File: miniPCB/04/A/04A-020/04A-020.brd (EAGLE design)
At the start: 41 parts

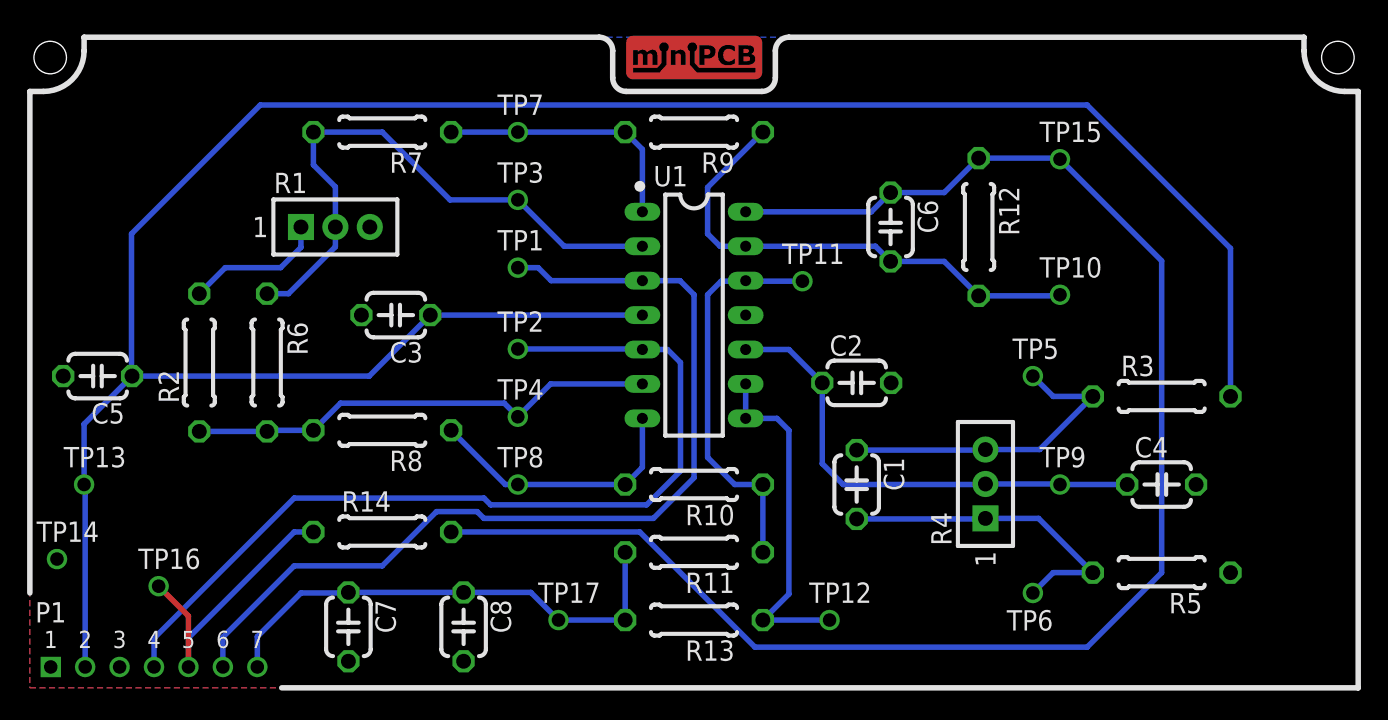
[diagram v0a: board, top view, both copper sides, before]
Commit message: NM.14JAN2023
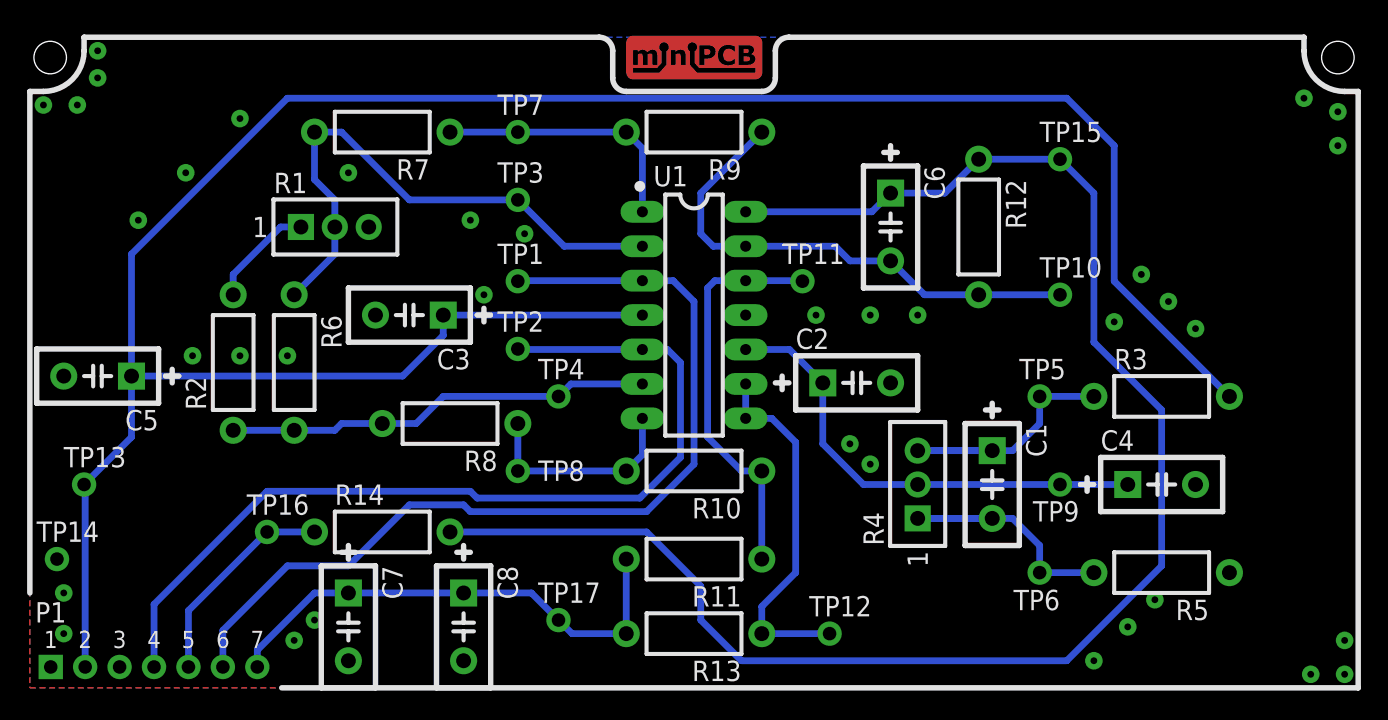
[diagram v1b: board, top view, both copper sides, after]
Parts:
- U1: value (none) -> OPAMP_QUADTHD
- moved C1 10.0 mm to (72.0, 16.0)
- moved TP16 8.94 mm to (18.5, 12.5)
- moved R8 5.02 mm to (32.0, 20.5)
- moved R4 5.00 mm to (66.5, 13.5)
- moved TP4 3.35 mm to (40.0, 22.5)
- moved R2 2.50 mm to (16.0, 25.0)
- moved R6 2.00 mm to (20.5, 25.0)
- moved TP5 1.58 mm to (75.5, 22.5)
- moved TP6 1.58 mm to (75.5, 9.50)
- moved C3 1.00 mm to (29.0, 28.5)
- moved R10 1.00 mm to (50.0, 17.0)
- moved R13 1.00 mm to (50.0, 5.00)
- moved TP1 1.00 mm to (37.0, 31.0)
- moved TP12 1.00 mm to (60.0, 5.00)
- moved TP8 1.00 mm to (37.0, 17.0)
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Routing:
- net N$11: track 21.5 -> 15.9 mm
- net N$8: track 19.9 -> 15.9 mm
- net N$6: track 35.0 -> 31.6 mm
- net POT.1: track 24.1 -> 21.3 mm
- net POT.3: track 24.1 -> 21.3 mm
- net N$10: track 10.4 -> 7.95 mm
- net OUT: track 116.7 -> 118.7 mm
- net N$5: track 43.4 -> 41.5 mm
- net N$9: track 25.8 -> 27.1 mm
- net N$4: track 69.6 -> 68.6 mm
- net N$3: track 66.9 -> 67.8 mm
- net BIAS: track 35.8 -> 35.0 mm
- net VFB: track 37.1 -> 37.7 mm
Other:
- board text added: "INSTRUMENTATION AMPLIFIER"

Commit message: NM.07MAR2024
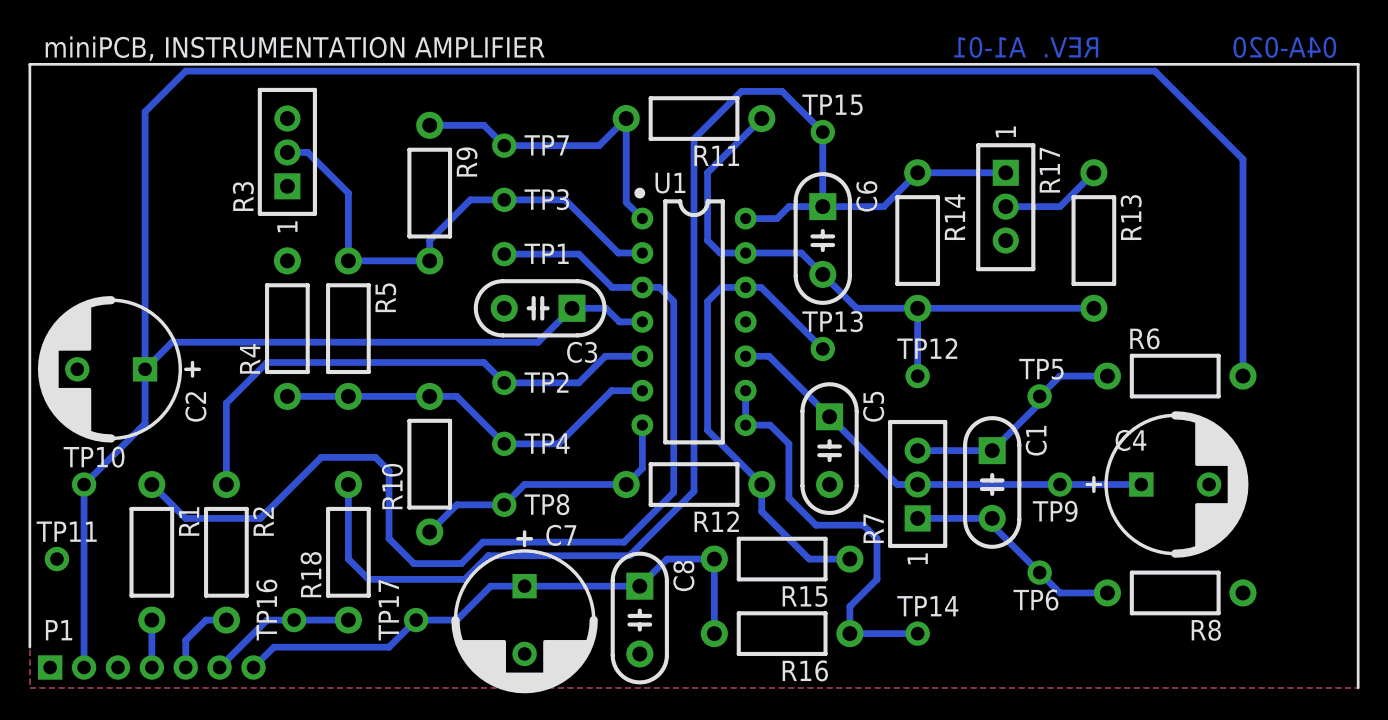
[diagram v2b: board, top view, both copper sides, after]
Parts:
- removed P1-: (no value), minipcb:MINIPCB_7P_50X100
- added P1: (no value), minipcb:PINS_1X7
- added R15, R16, R18: (no value), minipcb:0207/10
- added R17: (no value), minipcb:TRIM_0100
- added U2: CLASSIC-50X100, miniPCB_BOARDS:PCB50X100
- C2, C4, C7: device minipcb:C050-024X044 -> minipcb:C5MM
- R1, R4: device minipcb:TRIM_0100 -> minipcb:0207/10
- R3, R7: device minipcb:0207/10 -> minipcb:TRIM_0100
- U1: value OPAMP_QUADTHD -> (none)
- moved TP10 73.3 mm to (5.00, 16.0)
- moved R3 66.3 mm to (20.0, 38.0), turned to 90 degrees
- moved R6 65.0 mm to (85.5, 24.0), turned to 0 degrees
- moved TP14 63.7 mm to (66.5, 5.00)
- moved R5 62.6 mm to (24.5, 27.5), turned to 270 degrees
- moved TP11 58.7 mm to (3.00, 10.5)
- moved TP13 55.4 mm to (59.5, 26.0)
- moved C2 55.0 mm to (7.00, 24.5), turned to 180 degrees
- moved R8 54.9 mm to (85.5, 8.00)
- moved C5 54.3 mm to (60.0, 18.5), turned to 270 degrees
- moved R7 48.7 mm to (66.5, 13.5), turned to 90 degrees
- moved R4 48.6 mm to (20.0, 27.5)
- moved R14 45.0 mm to (66.5, 34.0), turned to 270 degrees
- moved R13 41.4 mm to (79.5, 34.0), turned to 270 degrees
- moved R11 32.5 mm to (50.0, 43.0)
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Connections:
- new net N$12: R13.1, R17.2
- new net N$13: P1.4, R1.2
- new net N$14: P1.5, R2.2
- net BIAS: now also C4.+, C5.1, R7.2; no longer C2.1, C4.1, R4.2
- net GND: now also C2.-, C4.-, C7.-, P1.1, R8.1, TP11.1; no longer C2.2, C4.2, C7.2, P1-.1, R5.1, TP14.1
- net N$1: now also R12.1, R15.1, TP13.1; no longer R10.1, R11.1, TP11.1
- net N$10: now also R3.1, R4.2; no longer R1.1, R2.2
- net N$11: now also P1.6, R18.1; no longer P1-.5, R14.1
- net N$2: now also C7.+, P1.7, R15.2, R16.2; no longer C7.1, P1-.7, R11.2, R13.2
- net N$3: now also R2.1; no longer P1-.4
- net N$4: now also R1.1; no longer P1-.6
- net N$5: now also R3.2, R5.1, R9.2; no longer R1.2, R6.1, R7.2
- net N$6: now also R10.2, R4.1, R5.2; no longer R2.1, R6.2, R8.2
- net N$7: now also R11.2, R9.1; no longer R7.1, R9.2
- net N$8: now also R10.1, R12.2; no longer R10.2, R8.1
- net N$9: now also R16.1, TP14.1; no longer R13.1, TP12.1
- net NC: now also P1.3; no longer P1-.3
- net OUT: now also R14.1, R17.1, R18.2; no longer R12.1, R14.2
- net POT.1: now also R7.1, R8.2; no longer R4.1, R5.2
- net POT.3: now also R6.1, R7.3; no longer R3.1, R4.3
- net V+: now also C2.+, P1.2, R6.2, TP10.1; no longer C5.1, P1-.2, R3.2, TP13.1
- net VFB: now also R11.1, R13.2, R14.2, TP12.1; no longer R12.2, R9.1, TP10.1
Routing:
- net N$3: track 67.8 -> 39.4 mm
- net OUT: track 118.7 -> 98.6 mm
- net V+: track 173.1 -> 182.8 mm
- net N$4: track 68.6 -> 77.8 mm
- net VFB: track 37.7 -> 46.2 mm
- net N$10: track 7.95 -> 0.00 mm
- net N$12: track 0.00 -> 7.54 mm
- net N$1: track 29.8 -> 35.9 mm
- net N$2: track 37.0 -> 42.8 mm
- net N$14: track 0.00 -> 5.62 mm
- net N$8: track 15.9 -> 20.8 mm
- net N$11: track 15.9 -> 10.9 mm
- net POT.3: track 21.3 -> 16.6 mm
- net POT.1: track 21.3 -> 16.6 mm
- net N$5: track 41.5 -> 36.8 mm
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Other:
- board text removed: "C1"
- board text removed: "C2"
- board text removed: "C3"
- board text removed: "C4"
- board text removed: "C5"
- board text removed: "C6"
- board text removed: "C7"
- board text removed: "C8"
- board text removed: "INSTRUMENTATION AMPLIFIER"
- board text removed: "R1"
- board text removed: "R10"
- board text removed: "R11"
- board text removed: "R12"
- board text removed: "R13"
- board text removed: "R14"
- board text removed: "R2"
- board text removed: "R3"
- board text removed: "R4"
- board text removed: "R5"
- board text removed: "R6"
- board text removed: "R7"
- board text removed: "R8"
- board text removed: "R9"
- board text removed: "TP1"
- board text removed: "TP10"
- board text removed: "TP11"
- board text removed: "TP12"
- board text removed: "TP13"
- board text removed: "TP14"
- board text removed: "TP15"
- board text removed: "TP16"
- board text removed: "TP17"
- board text removed: "TP2"
- board text removed: "TP3"
- board text removed: "TP4"
- board text removed: "TP5"
- board text removed: "TP6"
- board text removed: "TP7"
- board text removed: "TP8"
- board text removed: "TP9"
- board text removed: "U1"
